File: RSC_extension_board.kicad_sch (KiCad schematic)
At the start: 31 parts, among them J1 NPTC202KFMS-RC, J10 Conn_01x04, J11 Conn_01x03, J12 Conn_01x03, J13 Conn_01x10, J2 Conn_01x02, J3 Raspberry_Pi_4, J4 TSM-120-01-L-DH-A-K-TR, J5 Conn_01x02, J6 Conn_01x03, J7 Conn_01x03, J8 Conn_01x03, J9 PRT-14417, Q1 2N7002-7-F, Q2 BSS138

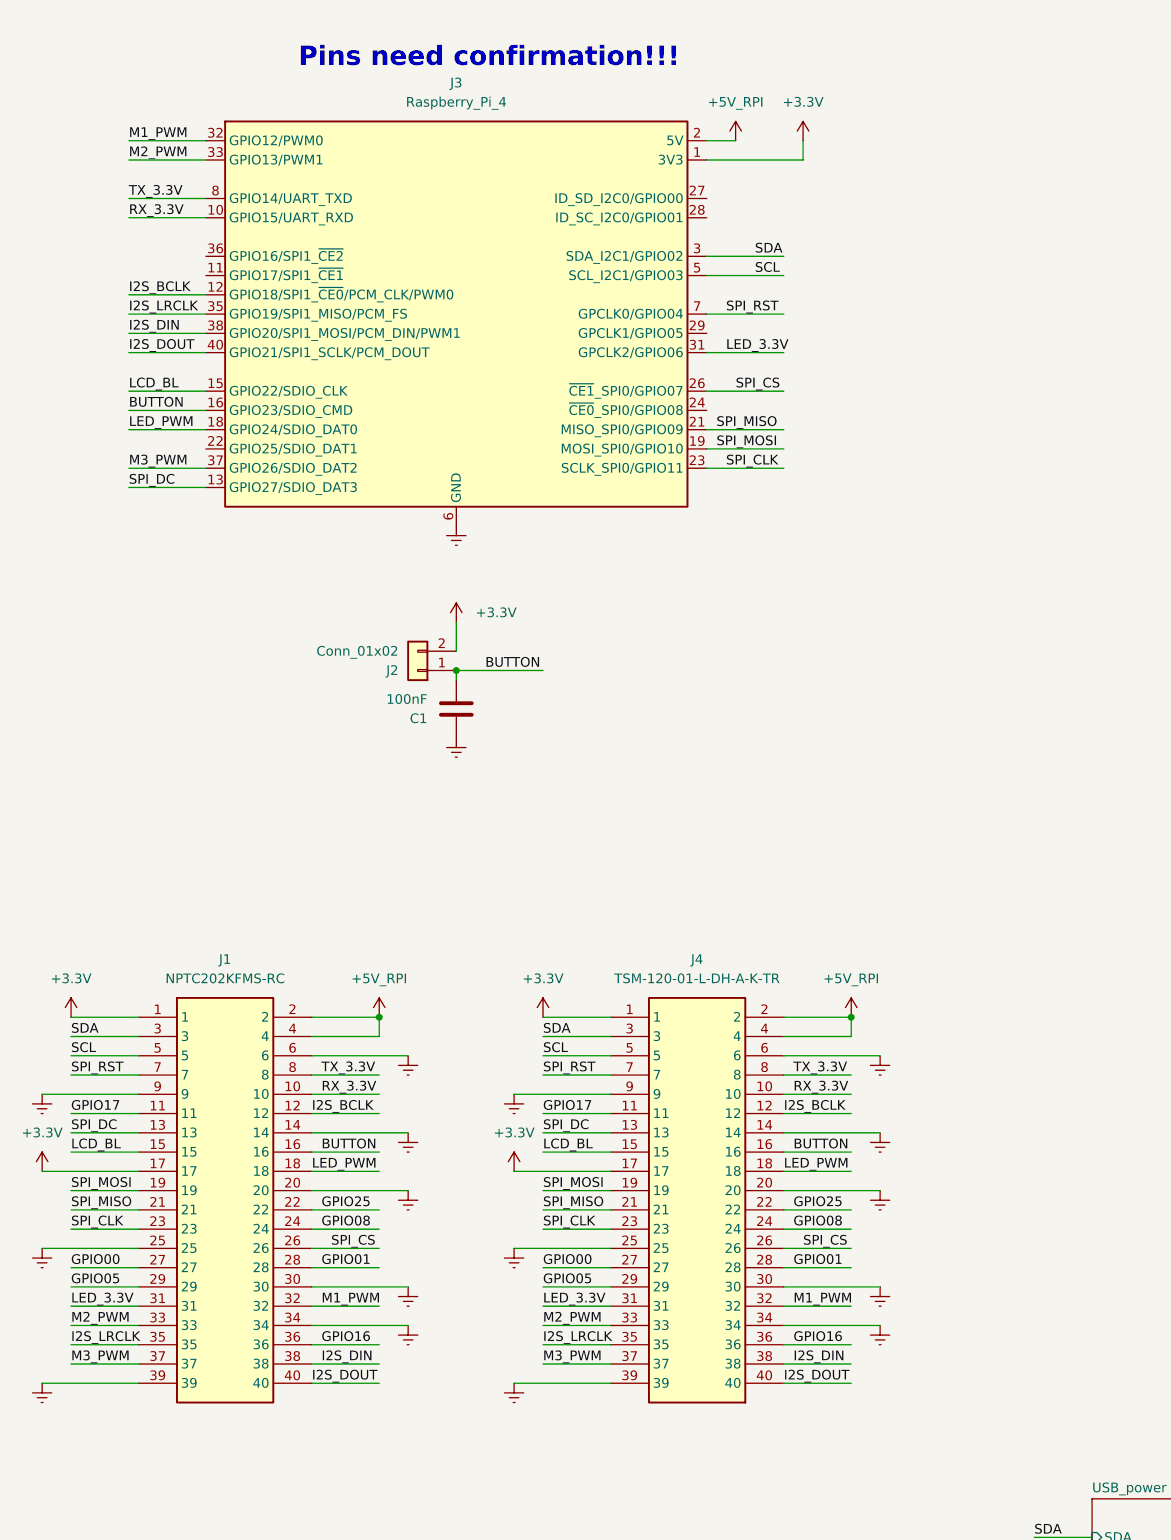
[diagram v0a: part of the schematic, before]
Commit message: silkscreen: logo, text, testpads.
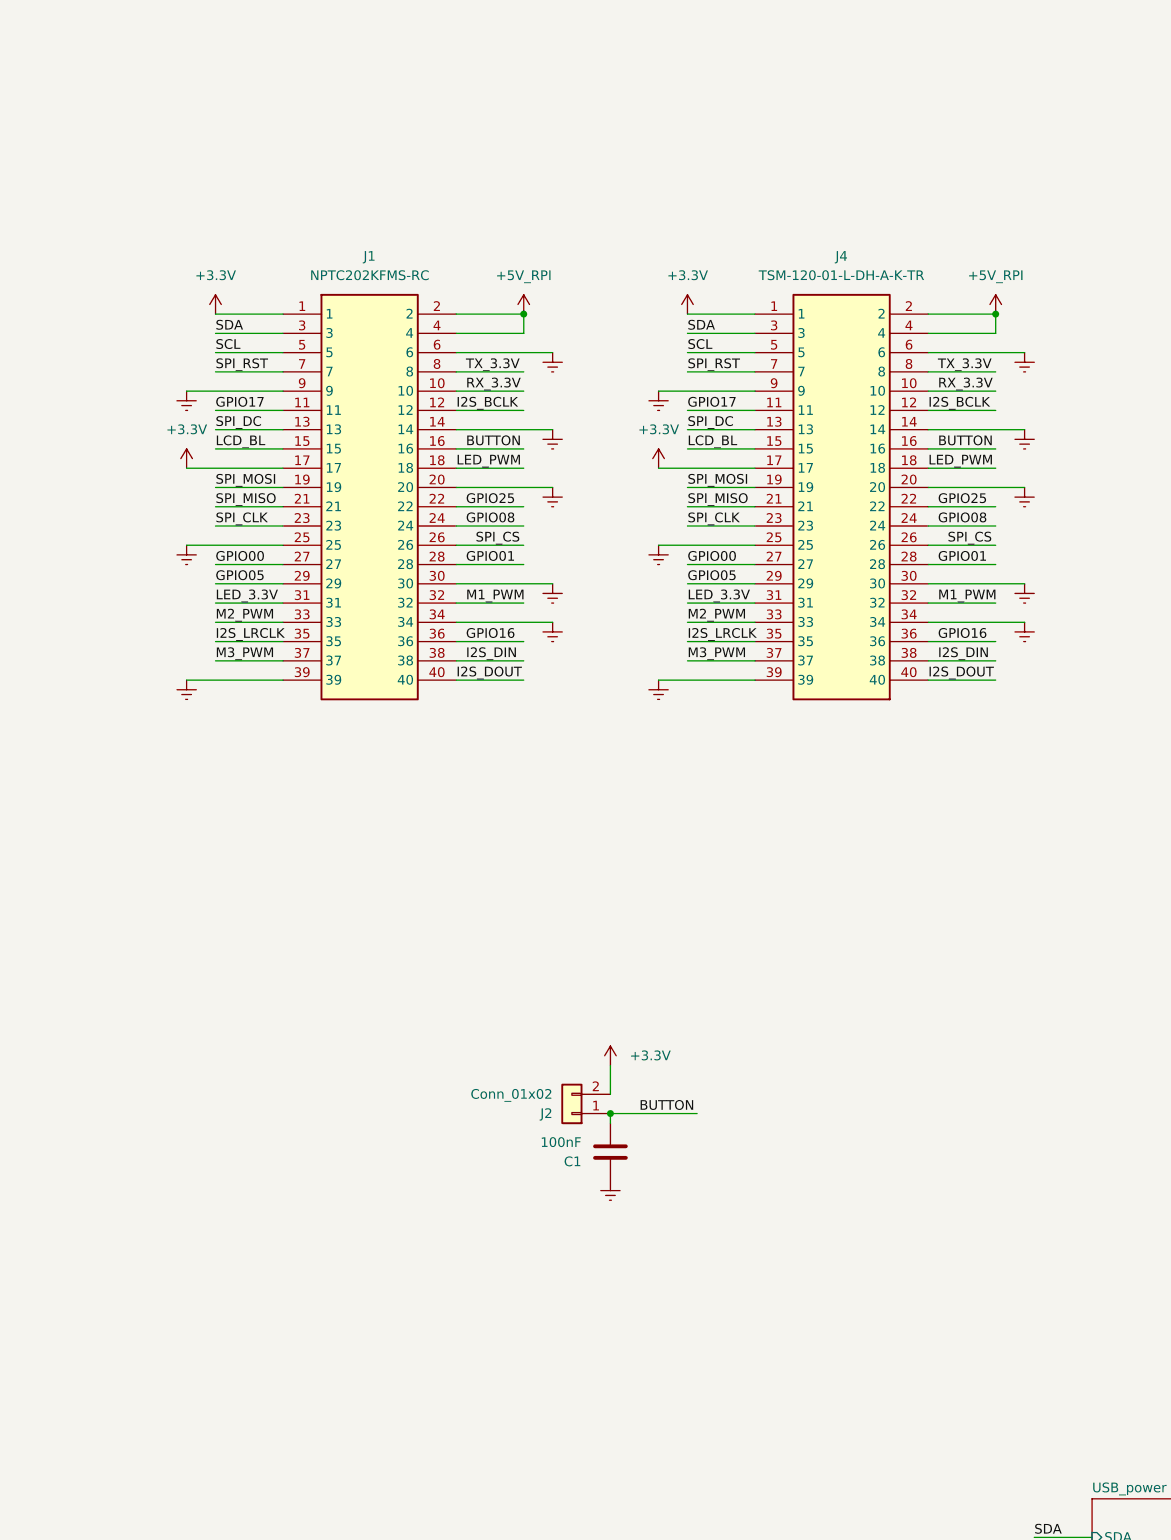
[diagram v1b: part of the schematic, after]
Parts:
- removed J3: Raspberry_Pi_4, KiCad:M207812045R_bottomLayer, symbol Connector:Raspberry_Pi_4
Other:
- note removed: "Pins need confirmation!!!"
- moved on the sheet: C1, J1, J2, J4
